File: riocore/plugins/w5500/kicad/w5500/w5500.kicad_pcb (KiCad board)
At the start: 2 copper layers, 52.2 x 21.8 mm, 34 parts, among them J6 RJ45_Pulse_J0011D21BNL, U8 W5500, Y2 Crystal_25MHz

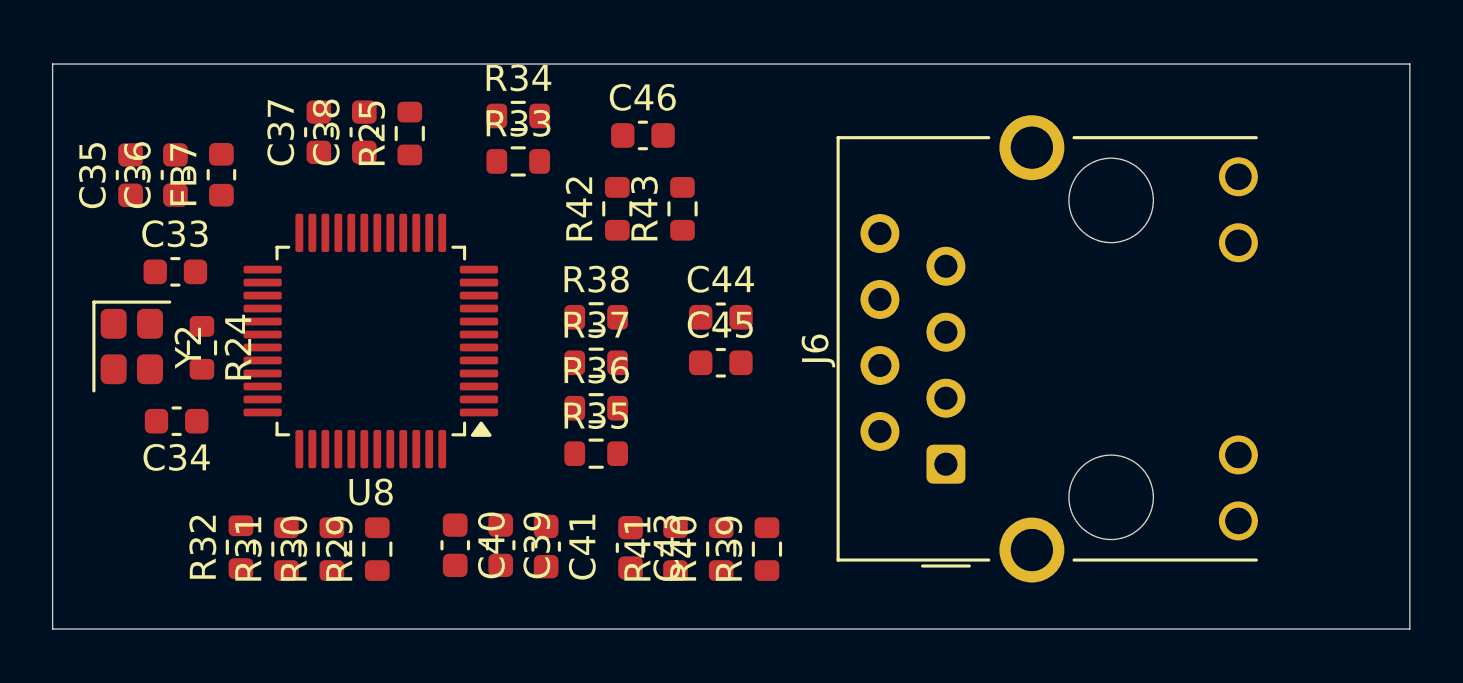
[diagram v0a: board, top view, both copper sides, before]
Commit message: kicad: fixes
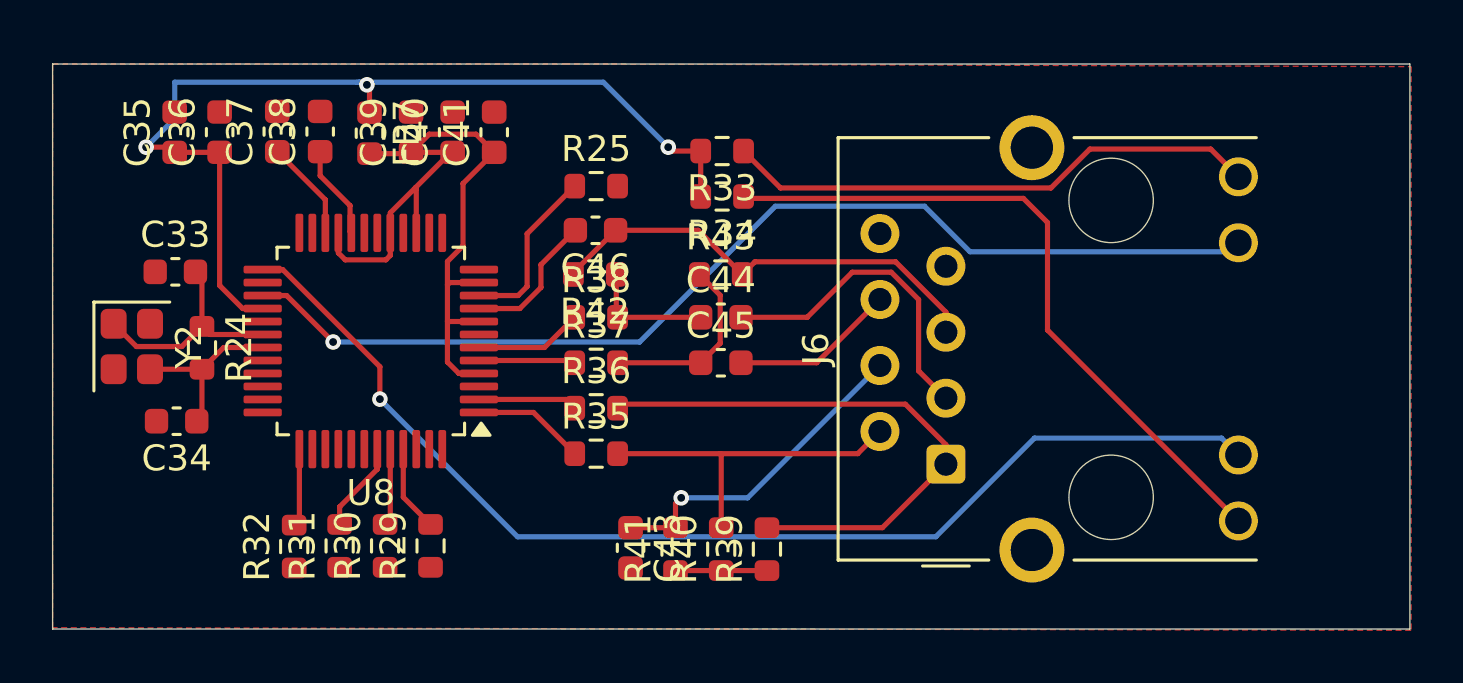
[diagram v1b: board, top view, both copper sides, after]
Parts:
- moved C39 16.3 mm to (140.3, 80.1), turned to 90 degrees
- moved C41 16.1 mm to (143.5, 80.1), turned to 90 degrees
- moved C40 15.9 mm to (141.9, 80.1), turned to 90 degrees
- moved R34 8.44 mm to (152.3, 82.6), turned to 180 degrees
- moved R33 7.86 mm to (152.3, 80.8), turned to 180 degrees
- moved R25 7.46 mm to (147.4, 82.2), turned to 0 degrees
- moved FB7 5.92 mm to (138.7, 80.2), turned to -90 degrees
- moved C46 4.08 mm to (147.4, 83.9), turned to 180 degrees
- moved R43 2.92 mm to (152.2, 85.6), turned to 0 degrees
- moved R42 2.67 mm to (147.4, 85.6), turned to 180 degrees
- moved C36 2.37 mm to (132.9, 80.1)
- moved C35 2.37 mm to (131.2, 80.1)
- moved R29 2.05 mm to (141.1, 96.0)
- moved R30 2.05 mm to (139.3, 96.0)
- moved R31 2.05 mm to (137.6, 96.0)
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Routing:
- net /LED_GRN: track 0.00 -> 44.4 mm, vias 0 -> 1
- net /LED_YEL: track 0.00 -> 41.3 mm, vias 0 -> 1
- net +3V3: track 0.00 -> 37.6 mm, vias 0 -> 3
- net /3V3_ADD: track 0.00 -> 32.9 mm
- net Net-(J6-Pad9): track 0.00 -> 26.6 mm
- net Net-(J6-TD+): track 0.00 -> 22.0 mm
- net Net-(J6-Pad12): track 0.00 -> 20.7 mm
- net Net-(J6-RCT): track 0.00 -> 17.6 mm
- net Net-(J6-TD-): track 0.00 -> 13.3 mm
- net Net-(J6-TCT): track 0.00 -> 12.7 mm, vias 0 -> 1
- net Net-(J6-RD+): track 0.00 -> 12.2 mm
- net Net-(U8-XI/CLKIN): track 0.00 -> 8.75 mm
- net Net-(C45-Pad1): track 0.00 -> 7.24 mm
- net Net-(U8-XO): track 0.00 -> 6.77 mm
- net Net-(U8-EXRES1): track 0.00 -> 6.62 mm
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- added copper zone on F.Cu, net GND

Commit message: kicad: some fixes
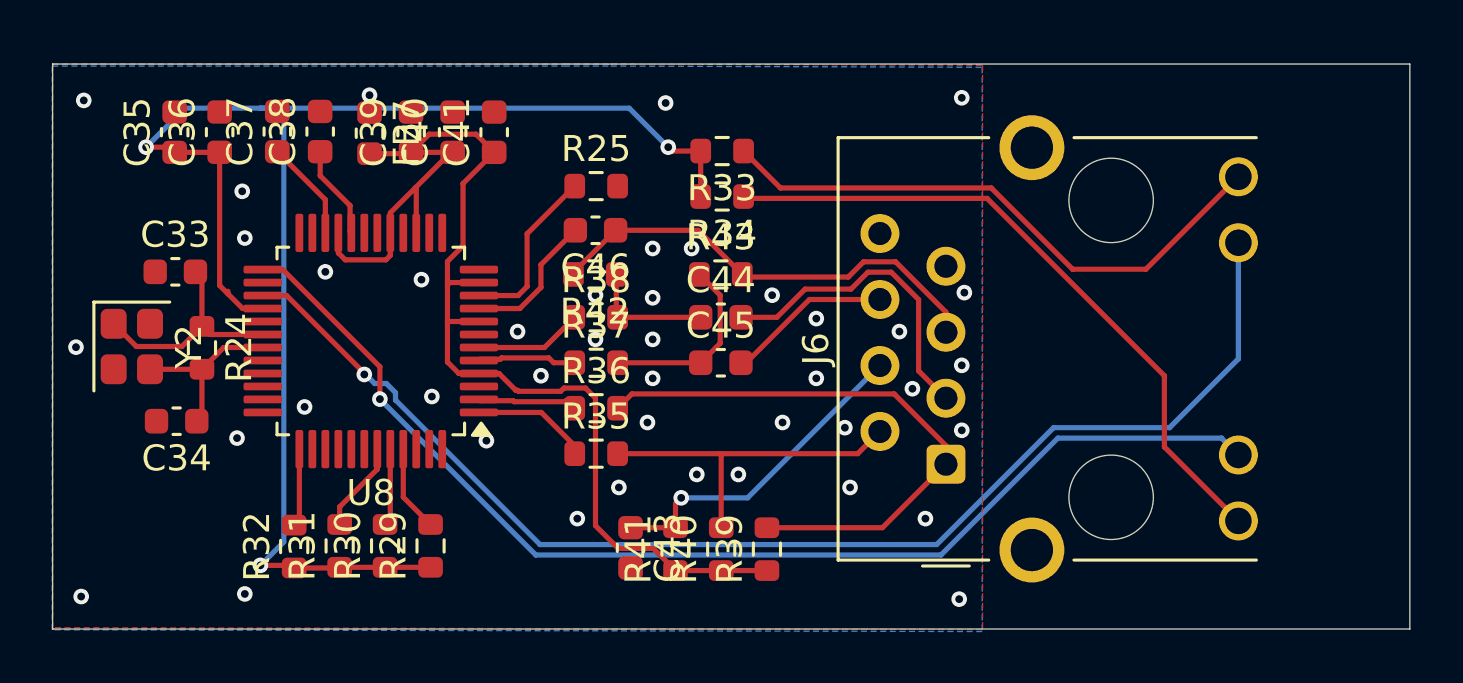
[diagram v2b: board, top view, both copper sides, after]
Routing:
- net +3V3: track 37.6 -> 60.6 mm, vias 3 -> 4
- net /3V3_ADD: track 32.9 -> 46.6 mm
- net /LED_YEL: track 41.3 -> 49.2 mm
- net Net-(J6-Pad12): track 20.7 -> 22.6 mm
- net Net-(J6-Pad9): track 26.6 -> 25.8 mm
- net /LED_GRN: track 44.4 -> 45.0 mm
- net GND: vias 0 -> 41
- added copper zone on B.Cu, net GND

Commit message: kicad: multiboard support
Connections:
- net /W5500.MISO renamed /miso
- net /W5500.MOSI renamed /mosi
- net /W5500.SCLK renamed /sclk
- net /W5500.nINT renamed /intr
- net /W5500.nRST renamed /rst
- net /W5500.nSCS renamed /sel
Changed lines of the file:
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@@
 	(net 16 "Net-(U8-PMODE1)")
 	(net 17 "Net-(U8-PMODE2)")
-	(net 18 "/W5500.nRST")
+	(net 18 "/rst")
 	(net 19 "Net-(J6-Pad12)")
 	(net 20 "Net-(J6-Pad9)")
@@
 	(net 30 "/LED_GRN")
 	(net 31 "unconnected-(U8-RSVD-Pad38)")
-	(net 32 "/W5500.MISO")
-	(net 33 "/W5500.SCLK")
+	(net 32 "/miso")
+	(net 33 "/sclk")
 	(net 34 "unconnected-(U8-DUPLED-Pad26)")
 	(net 35 "unconnected-(U8-RSVD-Pad42)")
@@
 	(net 40 "unconnected-(U8-RSVD-Pad41)")
 	(net 41 "unconnected-(U8-NC-Pad47)")
-	(net 42 "/W5500.nINT")
+	(net 42 "/intr")
 	(net 43 "unconnected-(U8-NC-Pad13)")
 	(net 44 "unconnected-(U8-NC-Pad12)")
-	(net 45 "/W5500.nSCS")
-	(net 46 "/W5500.MOSI")
+	(net 45 "/sel")
+	(net 46 "/mosi")
 	(net 47 "unconnected-(U8-RSVD-Pad40)")
 	(footprint "Resistor_SMD:R_0603_1608Metric"
@@
 			(layers "F.Cu" "F.Mask" "F.Paste")
 			(roundrect_rratio 0.25)
-			(net 45 "/W5500.nSCS")
+			(net 45 "/sel")
 			(pinfunction "~{SCS}")
 			(pintype "input")
@@
 			(layers "F.Cu" "F.Mask" "F.Paste")
 			(roundrect_rratio 0.25)
-			(net 33 "/W5500.SCLK")
+			(net 33 "/sclk")
 			(pinfunction "SCLK")
 			(pintype "input")
@@
 			(layers "F.Cu" "F.Mask" "F.Paste")
 			(roundrect_rratio 0.25)
-			(net 32 "/W5500.MISO")
+			(net 32 "/miso")
 			(pinfunction "MISO")
 			(pintype "output")
@@
 			(layers "F.Cu" "F.Mask" "F.Paste")
 			(roundrect_rratio 0.25)
-			(net 46 "/W5500.MOSI")
+			(net 46 "/mosi")
 			(pinfunction "MOSI")
 			(pintype "input")
@@
 			(layers "F.Cu" "F.Mask" "F.Paste")
 			(roundrect_rratio 0.25)
-			(net 42 "/W5500.nINT")
+			(net 42 "/intr")
 			(pinfunction "~{INT}")
 			(pintype "input")
@@
 			(layers "F.Cu" "F.Mask" "F.Paste")
 			(roundrect_rratio 0.25)
-			(net 18 "/W5500.nRST")
+			(net 18 "/rst")
 			(pinfunction "~{RST}")
 			(pintype "input")
@@
 			(at 0 1.43 90)
 			(layer "F.Fab")
+			(hide yes)
 			(effects
 				(font
@@
 			(layers "F.Cu" "F.Mask" "F.Paste")
 			(roundrect_rratio 0.25)
-			(net 18 "/W5500.nRST")
+			(net 18 "/rst")
 			(pintype "passive")
 		)
@@
 		)
 		(property "Value" "RJ45_Pulse_J0011D21BNL"
-			(at 4.44 18.5 90)
+			(at 4.44 15.71 90)
 			(layer "F.Fab")
 			(effects
@@
 		)
 		(property "Value" "10uF/6.3V"
-			(at 0 1.43 90)
+			(at -1.675 -1.9 90)
 			(layer "F.Fab")
+			(hide yes)
 			(effects
 				(font
@@
 			(at 0 1.43 90)
 			(layer "F.Fab")
+			(hide yes)
 			(effects
 				(font
@@
 			(at 0 2.2 90)
 			(layer "F.Fab")
+			(hide yes)
 			(effects
 				(font

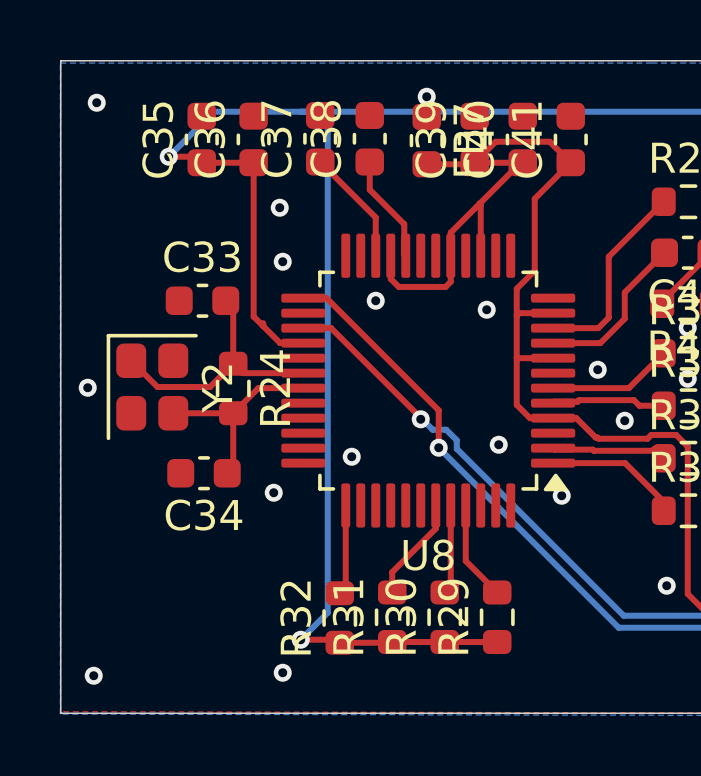
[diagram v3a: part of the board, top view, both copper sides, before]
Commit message: some changes
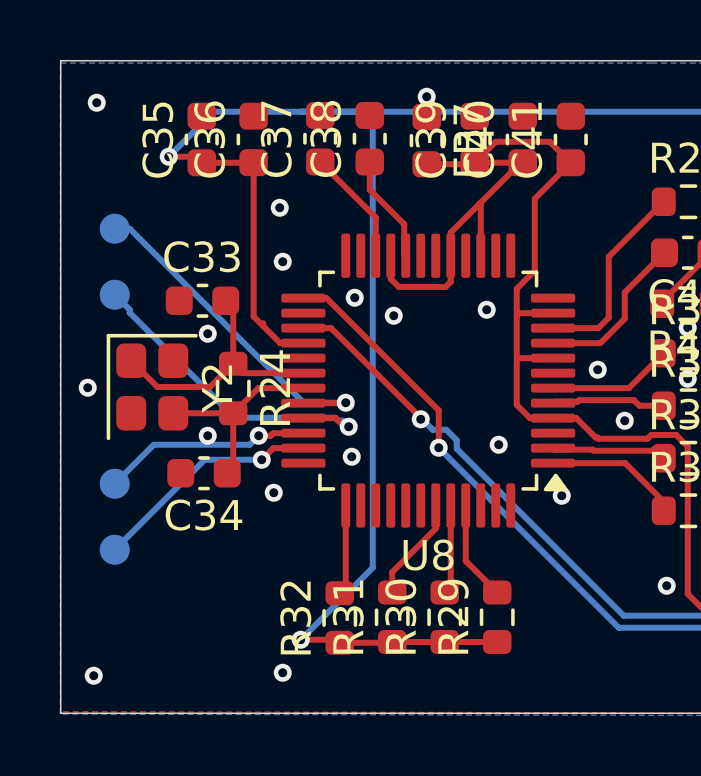
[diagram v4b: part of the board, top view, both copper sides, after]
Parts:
- added TP1: TestPoint, TestPoint:TestPoint_Pad_D1.0mm, B.Cu at (128.3, 83.1)
- added TP2: TestPoint, TestPoint:TestPoint_Pad_D1.0mm, B.Cu at (128.3, 85.3)
- added TP3: TestPoint, TestPoint:TestPoint_Pad_D1.0mm, B.Cu at (128.3, 91.6)
- added TP4: TestPoint, TestPoint:TestPoint_Pad_D1.0mm, B.Cu at (128.3, 93.8)
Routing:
- net /sel: track 0.00 -> 11.5 mm, vias 0 -> 1
- net /sclk: track 0.00 -> 11.3 mm, vias 0 -> 1
- net /mosi: track 0.00 -> 7.69 mm, vias 0 -> 1
- net /miso: track 0.00 -> 6.99 mm, vias 0 -> 1
- net +3V3: track 60.6 -> 62.7 mm
- net GND: vias 41 -> 44
